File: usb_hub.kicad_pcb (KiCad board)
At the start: 2 copper layers, 120 x 65 mm, 21 parts, among them J1 CONN_01X02_MALE-B2B, J10 USB_A, J11 USB_A, J12 USB_A, J13 USB_A, J14 USB_A, J15 USB_A, J16 USB_A, J17 USB_A, J18 CONN_COAXIAL, J19 CONN_COAXIAL, J2 CONN_01X02_MALE-B2B, J20 CONN_COAXIAL, J21 CONN_COAXIAL, J3 DIL24, J4 CONN_01X02_MALE, J5 CONN_01X02_MALE, J6 USB_A, J7 USB_A, J8 CONN_01X02_MALE, J9 CONN_01X02_MALE

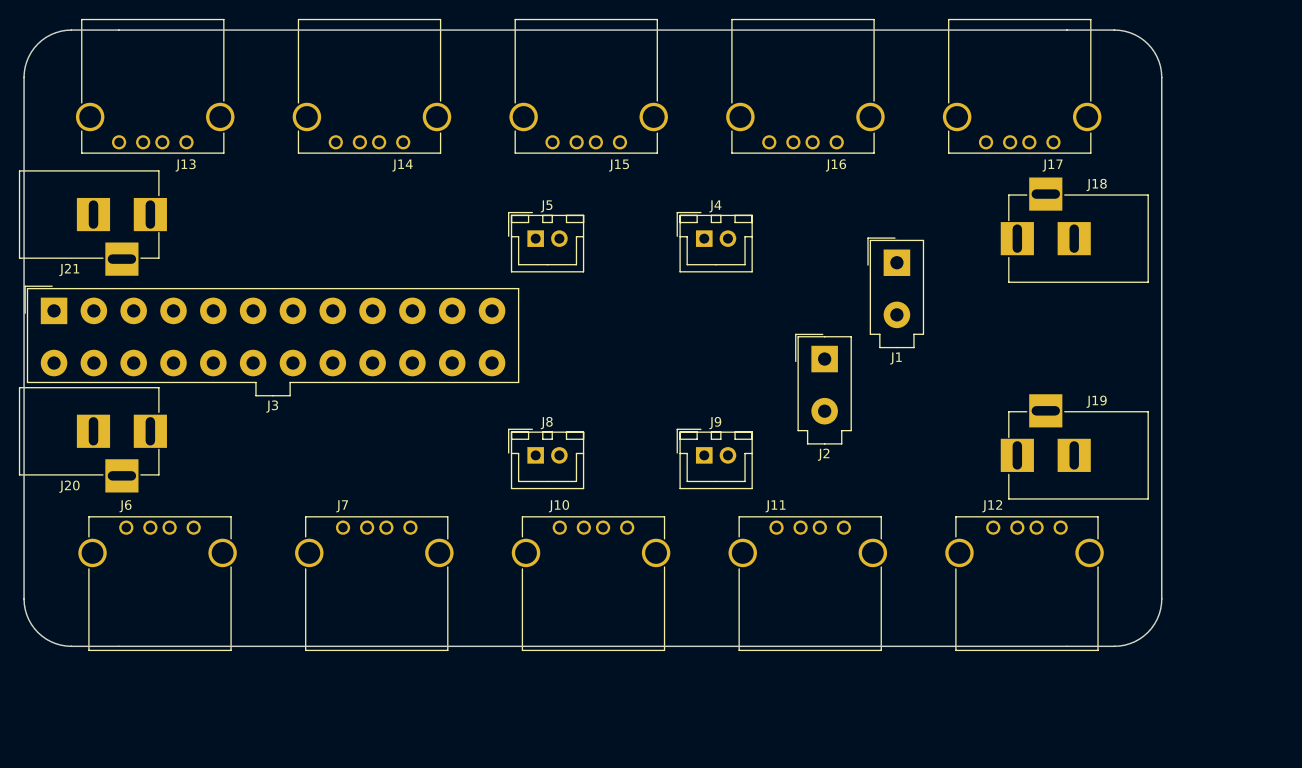
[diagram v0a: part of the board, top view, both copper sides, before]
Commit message: Rev A complete
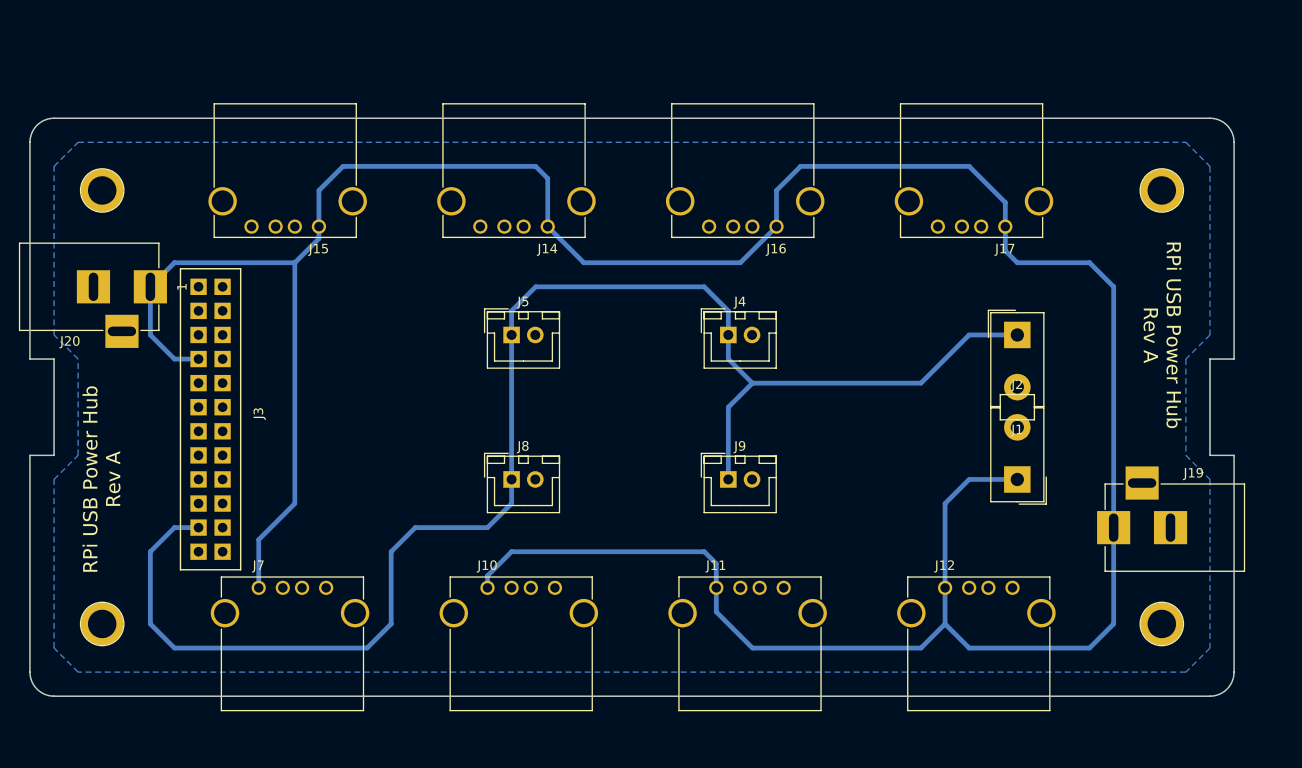
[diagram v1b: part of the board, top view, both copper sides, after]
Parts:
- removed J13, J6: USB_A, Connectors:USB_A
- removed J18, J21: CONN_COAXIAL, Connectors:BARREL_JACK
- added ?: 1pin, Connectors:1pin, F.Cu at (88.9, 71.9)
- added ?: 1pin, Connectors:1pin, F.Cu at (88.9, 117.6)
- added ?: 1pin, Connectors:1pin, F.Cu at (200.6, 117.6)
- added ?: 1pin, Connectors:1pin, F.Cu at (200.6, 71.9)
- J3: footprint Connectors_Molex:Molex_MiniFit-JR-5556-24A_2x12x4.20mm_Straight -> Custom_Connectors:ATX_Wire_On_Board
- moved J15 33.0 mm to (111.7, 75.7)
- moved J2 24.0 mm to (185.4, 102.4), turned to 180 degrees
- moved J14 17.6 mm to (135.9, 75.7)
- moved J3 16.6 mm to (95.9, 96.0), turned to 270 degrees
- moved J20 15.2 mm to (94.0, 82.1)
- moved J1 14.8 mm to (185.4, 87.2)
- moved J19 12.7 mm to (195.6, 107.5)
- moved J16 10.9 mm to (160.0, 75.7)
- moved J7 10.9 mm to (105.4, 113.8)
- moved J4 10.5 mm to (154.9, 87.2)
- moved J5 10.5 mm to (132.1, 87.2)
- moved J17 10.2 mm to (184.1, 75.7)
- moved J10 9.92 mm to (129.5, 113.8)
- moved J11 8.98 mm to (153.7, 113.8)
- moved J12 8.13 mm to (177.8, 113.8)
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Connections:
- J2 pad 1: GND -> +5V
- J2 pad 2: +5V -> GND
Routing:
- net +5V: track 0.00 -> 314.4 mm
- net +12V: track 0.00 -> 158.9 mm
- added copper zone on B.Cu, net GND
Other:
- board size 120 x 65 mm -> 127 x 61 mm
- net class Default: trace_width 0.25 -> 0.5
- board text added: "RPi USB Power Hub Rev A"
